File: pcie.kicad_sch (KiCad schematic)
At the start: 20 parts, among them U15 XC7K160T-FFG676

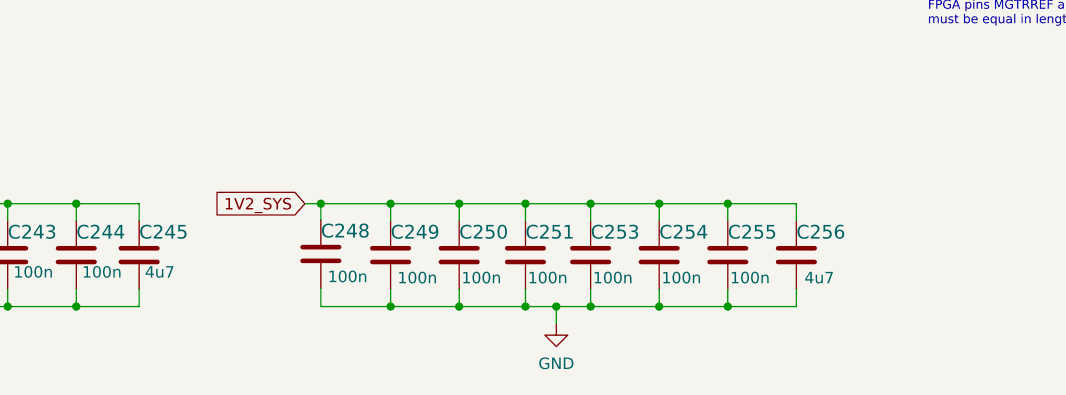
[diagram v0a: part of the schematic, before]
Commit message: Final touches
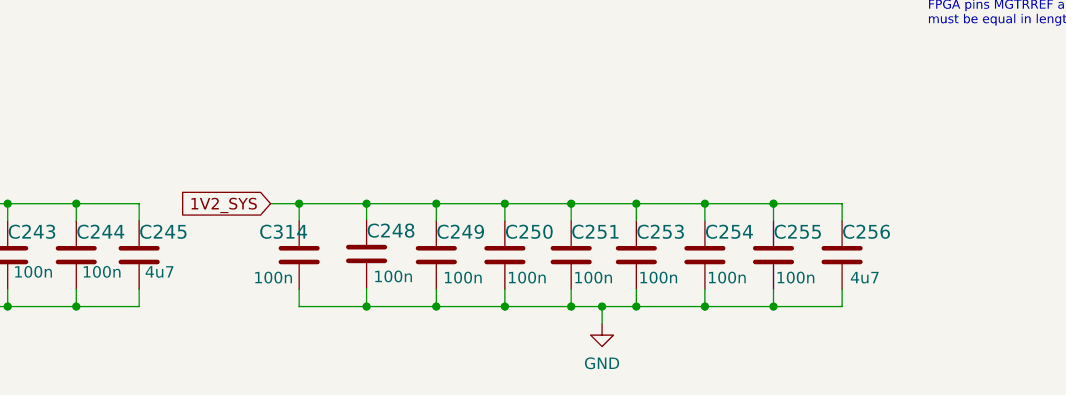
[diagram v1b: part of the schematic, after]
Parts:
- added C314: C_100n_0402, antmicro-footprints:0402-cap, symbol antmicroCapacitors0402:C_100n_0402
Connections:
- net 1V2_SYS: now also C314.1
- net GND: now also C314.2
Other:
- moved on the sheet: C248, C249, C250, C251, C253, C254, C255, C256
